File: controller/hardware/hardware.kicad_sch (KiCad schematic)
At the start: 28 parts, among them J1 Screw_Terminal_01x02, J2 Screw_Terminal_01x02, J3 Screw_Terminal_01x02, M1 HC-12, U1 TLV1117-33, U2 ESP32-C6-SuperMini, U3 MAX3485

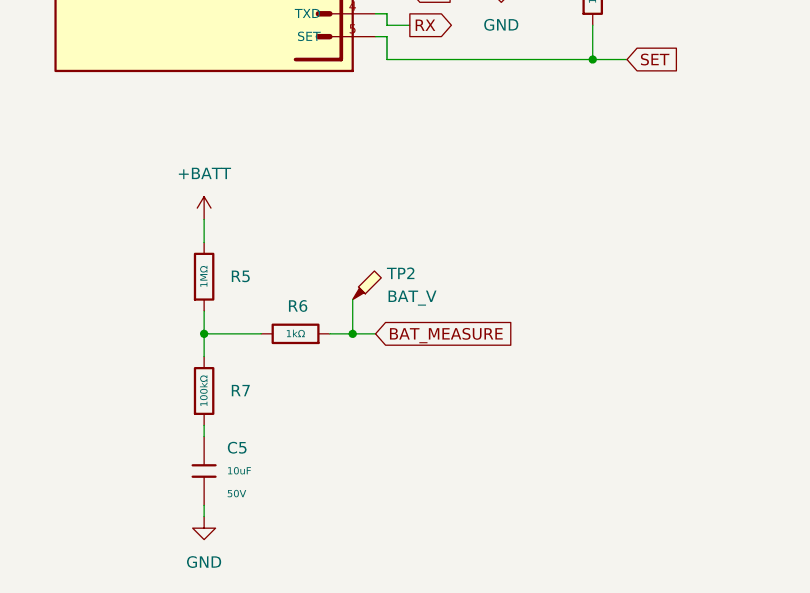
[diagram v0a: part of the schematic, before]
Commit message: final v1.0 hardware
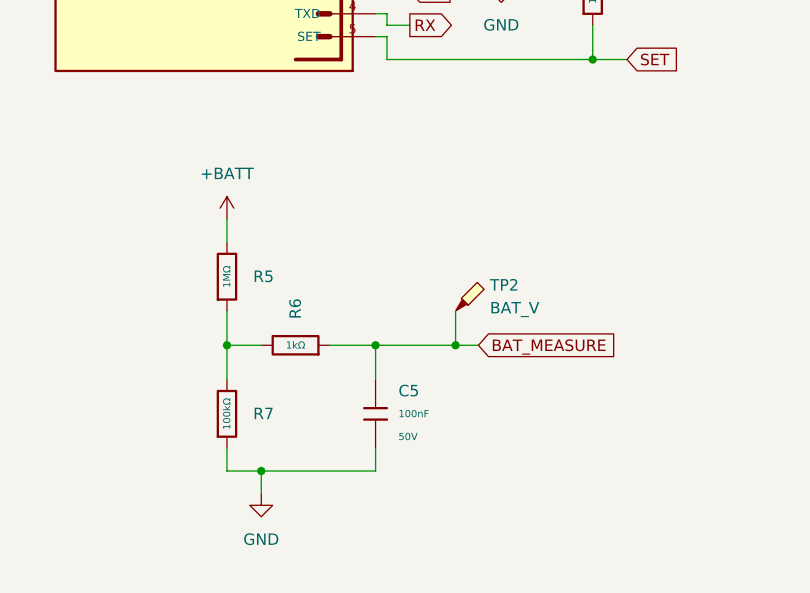
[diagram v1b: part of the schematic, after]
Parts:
- C5: value 10uF -> 100nF
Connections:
- net BAT_MEASURE: now also C5.2
- net GND: now also R7.1
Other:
- moved on the sheet: C5, R5, R6, R7, TP2
